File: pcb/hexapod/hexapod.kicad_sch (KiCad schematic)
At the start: 19 parts, among them J1 Conn_01x03, J10 Conn_01x03, J11 Conn_01x03, J12 Conn_01x03, J13 Conn_01x03, J14 Conn_01x03, J15 Conn_01x03, J16 Conn_01x03, J17 Conn_01x03, J18 Conn_01x03, J2 Conn_01x03, J3 Conn_01x03, J4 Conn_01x03, J5 Conn_01x03, J6 Conn_01x03, J7 Conn_01x03, J8 Conn_01x03, J9 Conn_01x03, U1 Pico

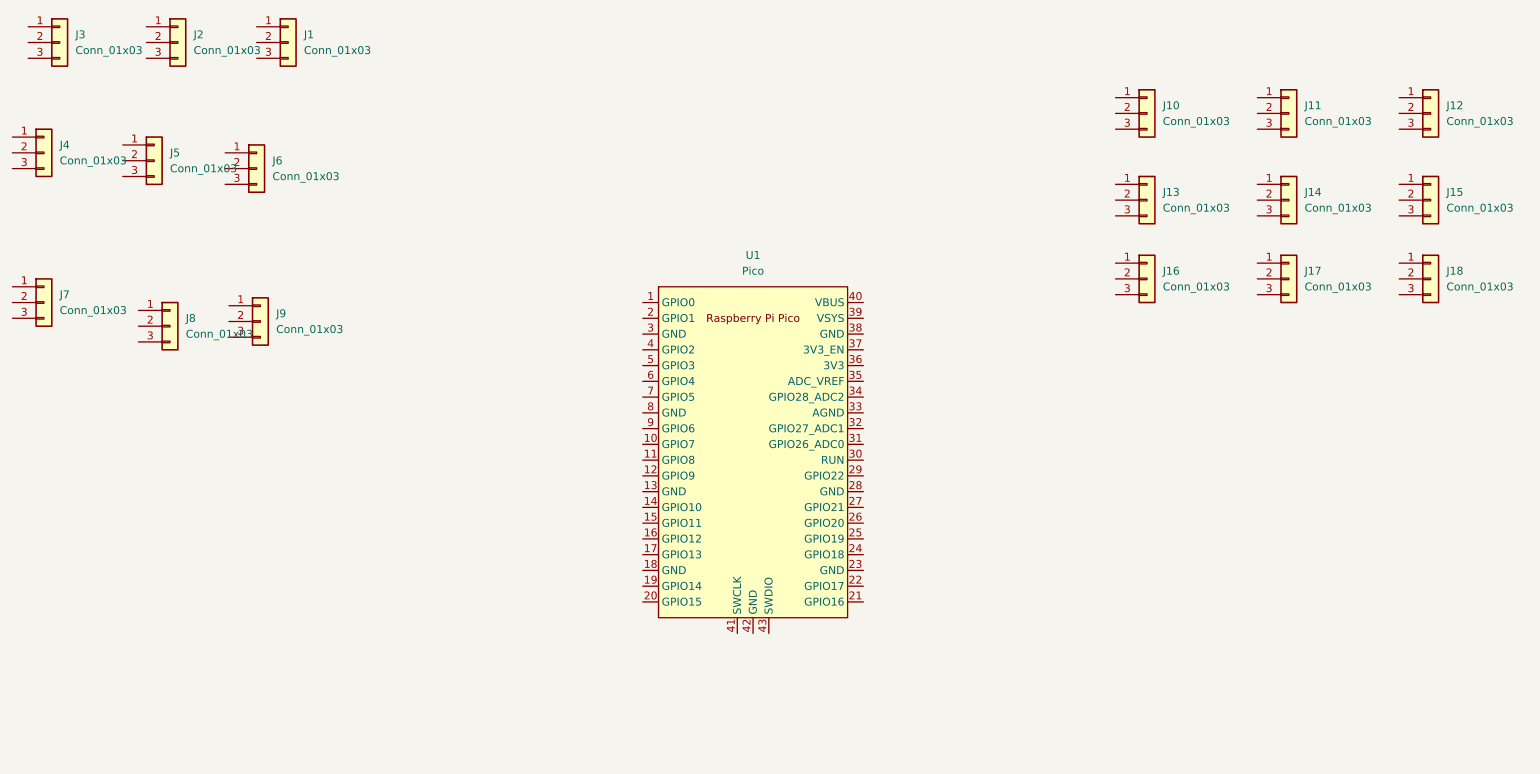
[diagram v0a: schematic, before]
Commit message: update
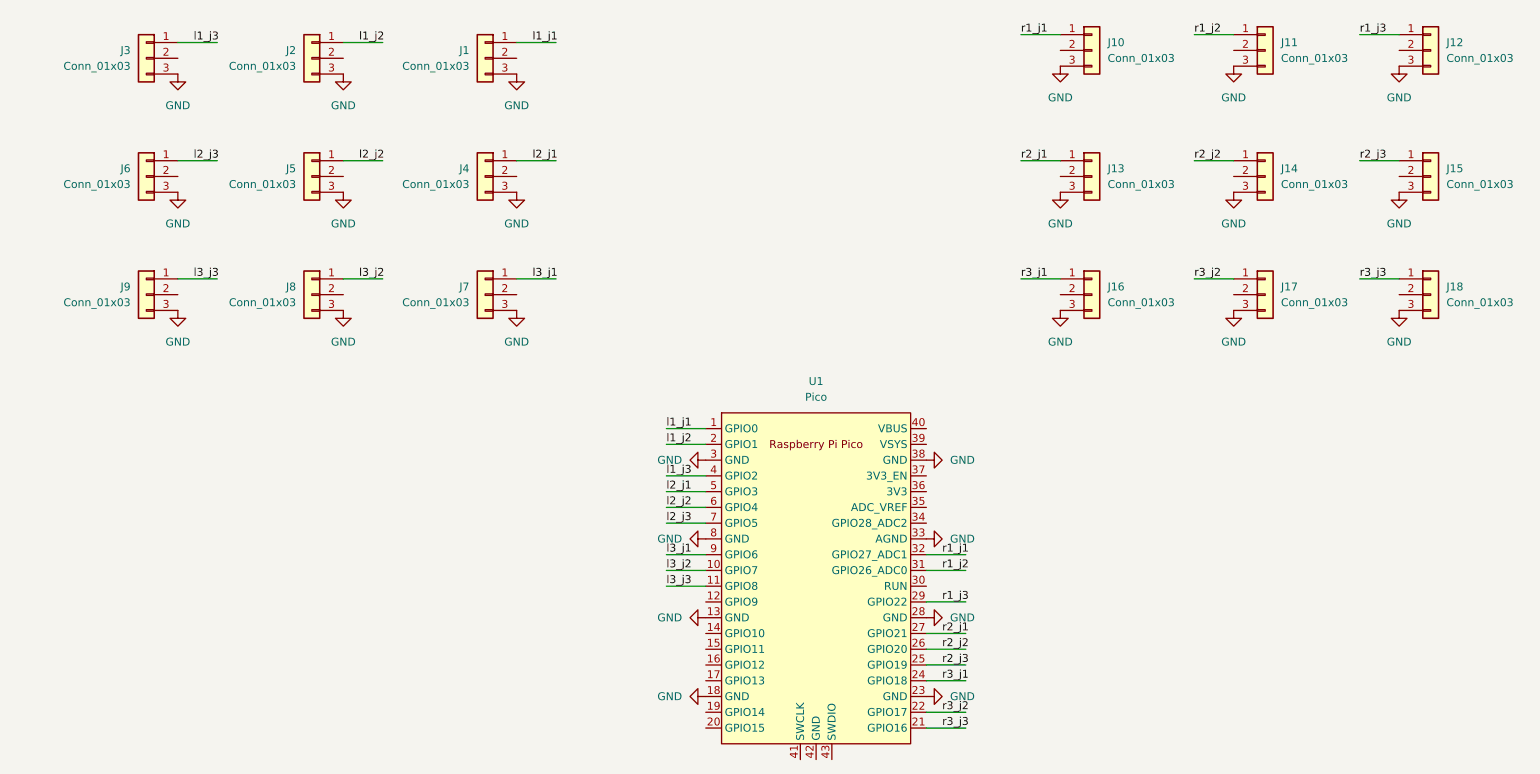
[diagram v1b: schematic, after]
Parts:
- U1: footprint RPi_Pico:RPi_Pico_SMD_TH -> RPi_Pico_SMD_TH
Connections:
- net l2_j2: now reaches J5.1 (Pin_1)
- net l2_j2: now also U1.6 (GPIO4)
- net GND: now reaches J5.3 (Pin_3)
- net GND: now also J1.3 (Pin_3), J10.3 (Pin_3), J11.3 (Pin_3), J12.3 (Pin_3), J13.3 (Pin_3), J14.3 (Pin_3), J15.3 (Pin_3), J16.3 (Pin_3), J17.3 (Pin_3), J18.3 (Pin_3), J2.3 (Pin_3), J3.3 (Pin_3), J4.3 (Pin_3), J6.3 (Pin_3), J7.3 (Pin_3), J8.3 (Pin_3), J9.3 (Pin_3), U1.13 (GND), U1.18 (GND), U1.23 (GND), U1.28 (GND), U1.3 (GND), U1.33 (AGND), U1.38 (GND), U1.8 (GND)
- net r3_j1: now reaches J16.1 (Pin_1)
- net r3_j1: now also U1.24 (GPIO18)
- net r2_j3: now reaches J15.1 (Pin_1)
- net r2_j3: now also U1.25 (GPIO19)
- net l1_j1: now reaches U1.1 (GPIO0)
- net l1_j1: now also J1.1 (Pin_1)
- net l3_j2: now reaches U1.10 (GPIO7)
- net l3_j2: now also J8.1 (Pin_1)
- net l3_j3: now reaches U1.11 (GPIO8)
- net l3_j3: now also J9.1 (Pin_1)
- net l1_j2: now reaches U1.2 (GPIO1)
- net l1_j2: now also J2.1 (Pin_1)
- net r3_j3: now reaches U1.21 (GPIO16)
- net r3_j3: now also J18.1 (Pin_1)
- net r3_j2: now reaches U1.22 (GPIO17)
- net r3_j2: now also J17.1 (Pin_1)
- net r2_j2: now reaches U1.26 (GPIO20)
- net r2_j2: now also J14.1 (Pin_1)
- net r2_j1: now reaches U1.27 (GPIO21)
- net r2_j1: now also J13.1 (Pin_1)
- net r1_j3: now reaches U1.29 (GPIO22)
- net r1_j3: now also J12.1 (Pin_1)
- net r1_j2: now reaches U1.31 (GPIO26_ADC0)
- net r1_j2: now also J11.1 (Pin_1)
- net r1_j1: now reaches U1.32 (GPIO27_ADC1)
- net r1_j1: now also J10.1 (Pin_1)
- net l1_j3: now reaches U1.4 (GPIO2)
- net l1_j3: now also J3.1 (Pin_1)
- net l2_j1: now reaches U1.5 (GPIO3)
- net l2_j1: now also J4.1 (Pin_1)
- net l2_j3: now reaches U1.7 (GPIO5)
- net l2_j3: now also J6.1 (Pin_1)
- net l3_j1: now reaches U1.9 (GPIO6)
- net l3_j1: now also J7.1 (Pin_1)
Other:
- moved on the sheet: J1, J10, J11, J12, J13, J14, J15, J16, J17, J18, J2, J3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
